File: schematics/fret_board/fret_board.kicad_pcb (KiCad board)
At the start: 2 copper layers, 1 part

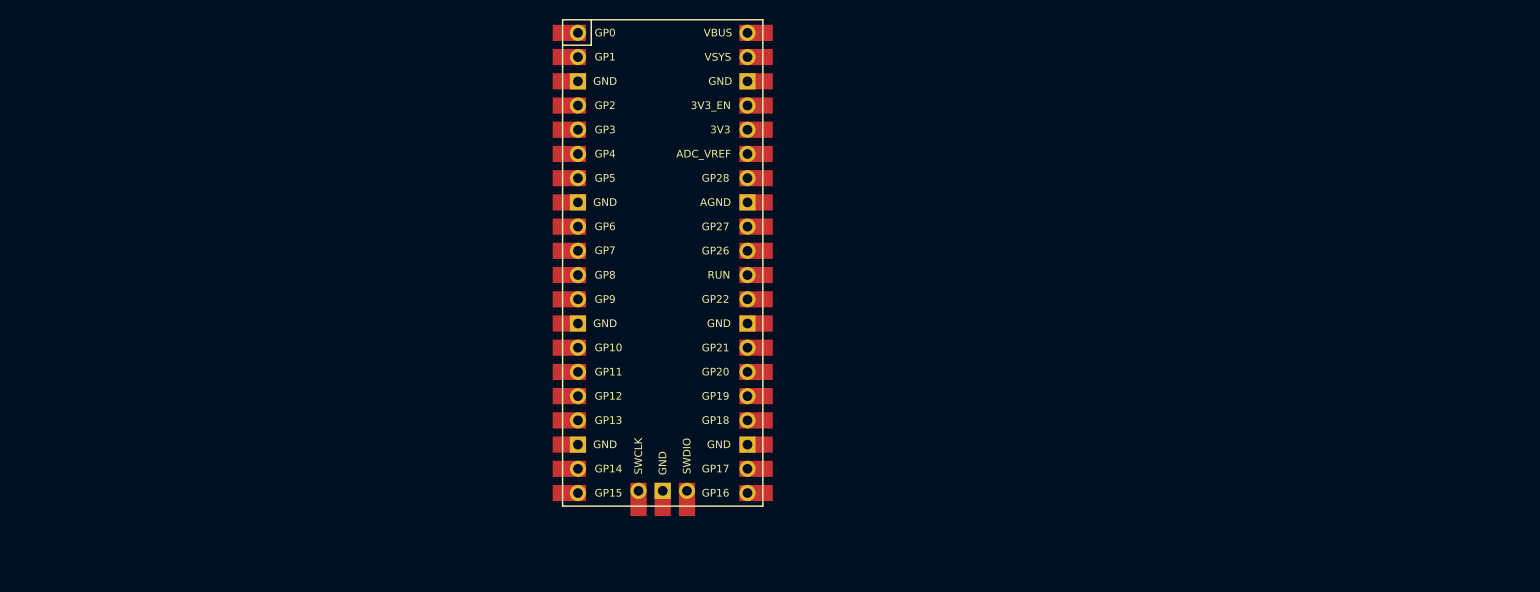
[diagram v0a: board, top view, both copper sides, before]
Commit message: Added schematic and PCB design to fret_board
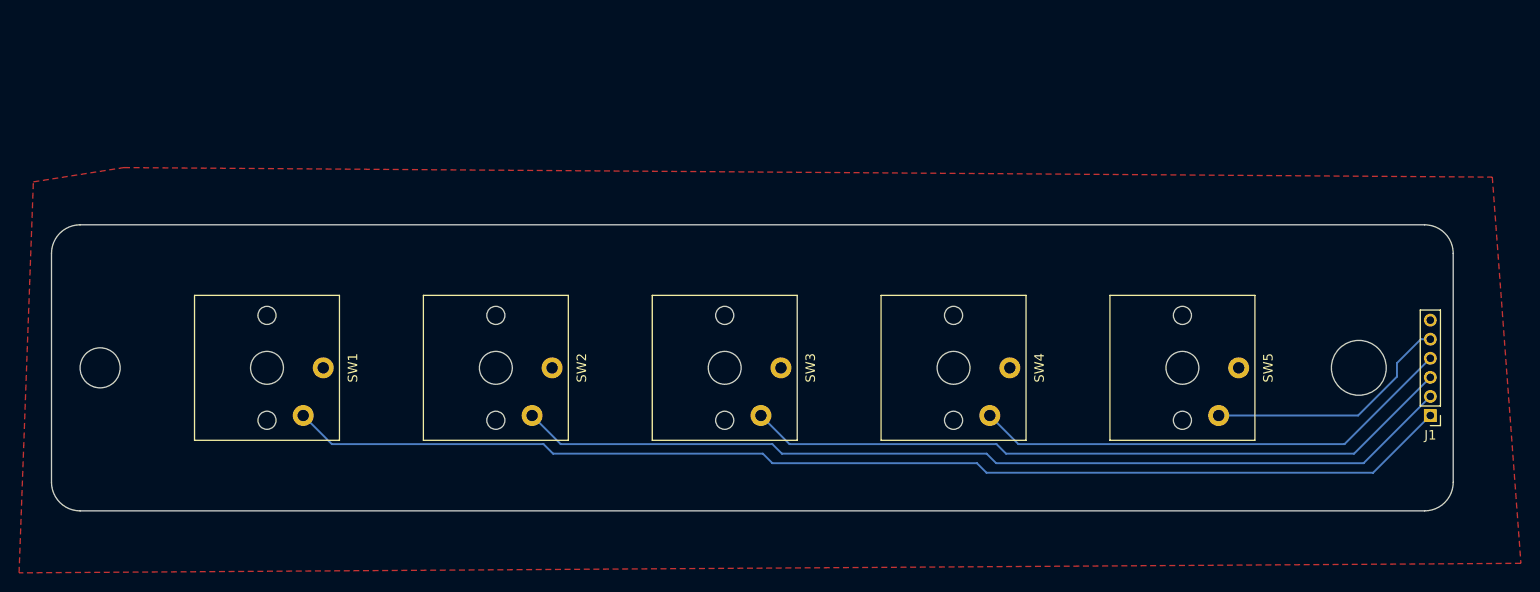
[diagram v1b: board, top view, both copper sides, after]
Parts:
- removed REF**: Raspberry_Pi_Pico, ScottoKeebs_MCU:Raspberry_Pi_Pico
- added J1: Conn_01x06, Connector_PinHeader_2.00mm:PinHeader_1x06_P2.00mm_Vertical, F.Cu at (225.5, 104.5)
- added SW1: Green, ScottoKeebs_Choc:Choc_V1, F.Cu at (103.5, 99.5)
- added SW2: Red, ScottoKeebs_Choc:Choc_V1, F.Cu at (127.5, 99.5)
- added SW3: Yellow, ScottoKeebs_Choc:Choc_V1, F.Cu at (151.5, 99.5)
- added SW4: Blue, ScottoKeebs_Choc:Choc_V1, F.Cu at (175.5, 99.5)
- added SW5: Orange, ScottoKeebs_Choc:Choc_V1, F.Cu at (199.5, 99.5)
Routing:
- net Net-(J1-Pin_1): track 0.00 -> 123.2 mm
- net Net-(J1-Pin_2): track 0.00 -> 99.2 mm
- net Net-(J1-Pin_3): track 0.00 -> 75.2 mm
- net Net-(J1-Pin_4): track 0.00 -> 51.2 mm
- net Net-(J1-Pin_5): track 0.00 -> 26.3 mm
- added copper zone on F.Cu, net GND
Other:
- board outline added: 147 x 30 mm
